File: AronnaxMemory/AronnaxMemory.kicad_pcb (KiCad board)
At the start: 6 copper layers, 161.3 x 64.8 mm, 38 parts, among them J1 Barrel_Jack_Switch, J11 Conn_02x18_Odd_Even, J2 Conn_02x40_Odd_Even, J3 Conn_02x18_Odd_Even, J8 RAM Select, J9 VP A1-A4, U10 AS6C4008-55PCN, U11 AS6C4008-55PCN, U12 AS6C4008-55PCN, U2 ATF22V10, U3 ATF22V10, U4 74AHCT32, U5 74HC74, U8 74HC74, U9 AS6C4008-55PCN, X1 16MHz

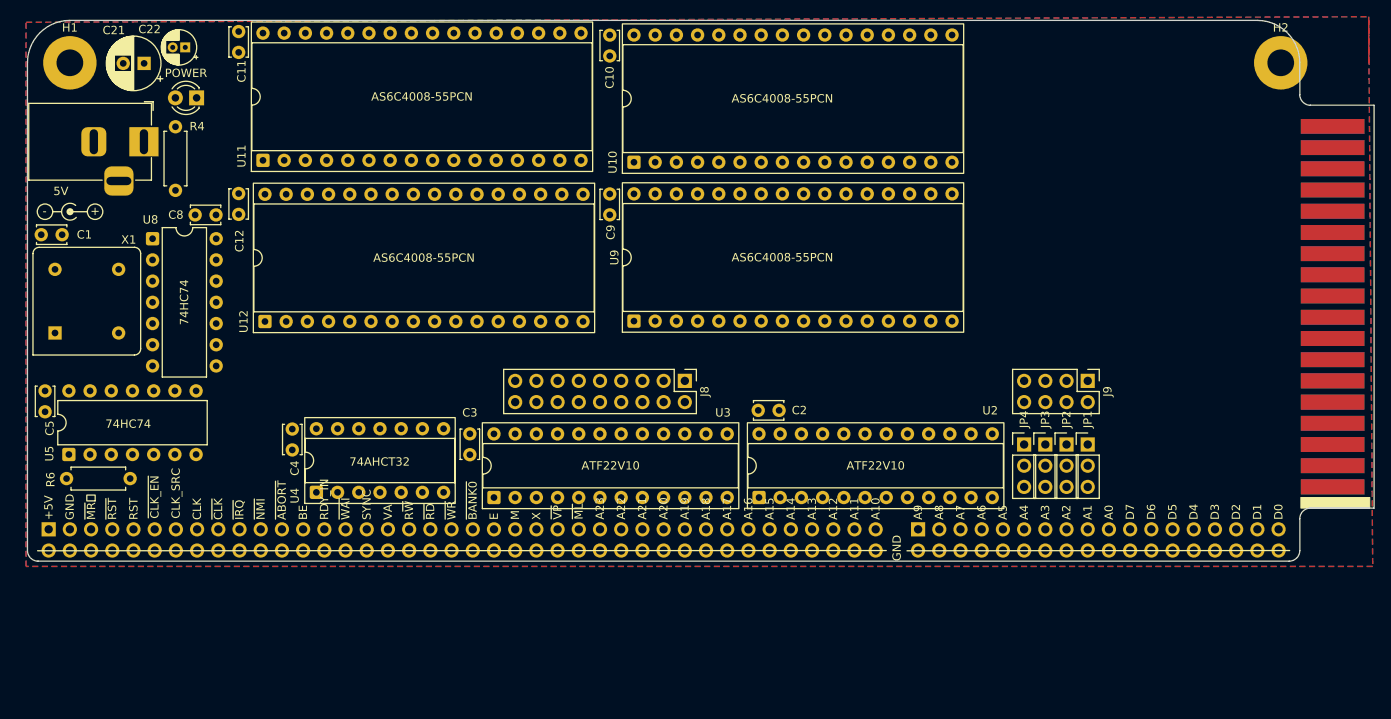
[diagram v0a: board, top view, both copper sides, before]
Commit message: May 2025
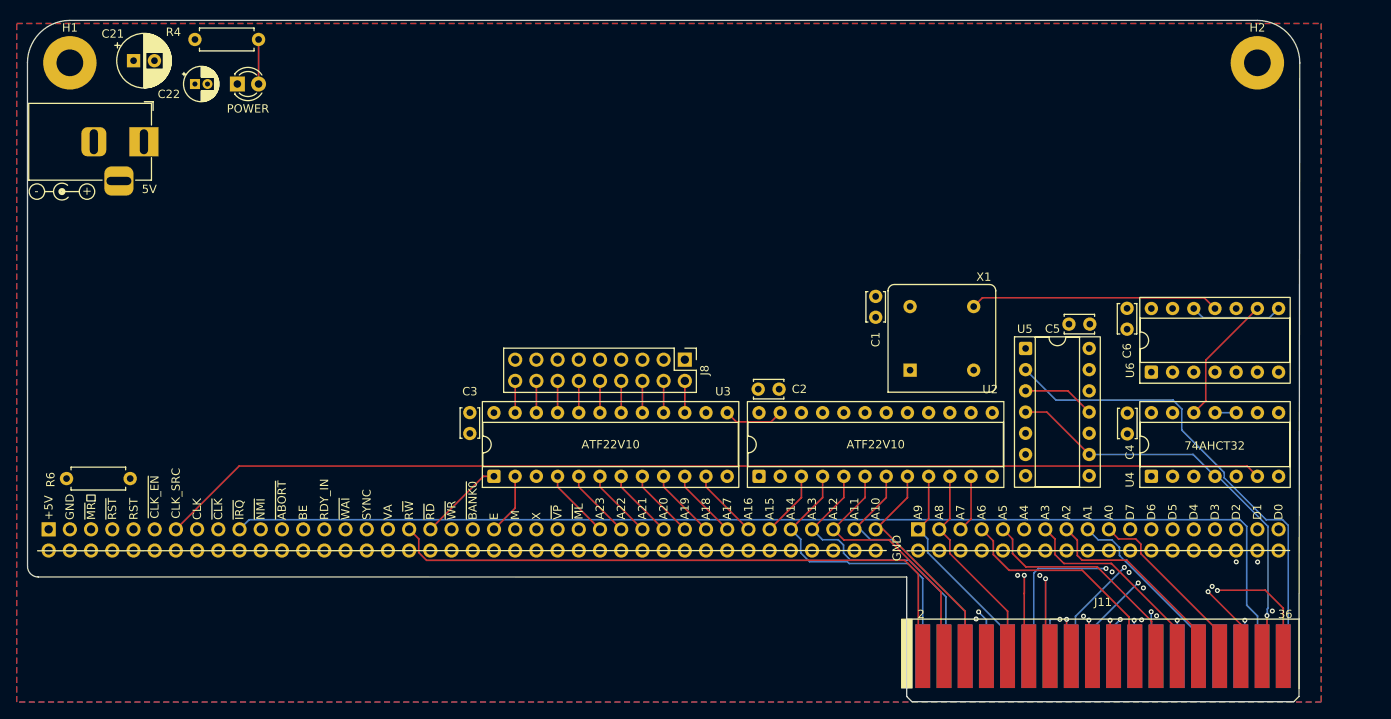
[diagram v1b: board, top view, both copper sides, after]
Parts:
- removed C10, C11, C12, C8, C9: 100nF, Capacitor_THT:C_Disc_D3.4mm_W2.1mm_P2.50mm
- removed J9: VP A1-A4, Connector_PinHeader_2.54mm:PinHeader_2x04_P2.54mm_Vertical
- removed JP1, JP2, JP3, JP4: Jumper3_254mm, Jumper3_254mm:Jumper3_254mm
- removed U10, U11, U12, U9: AS6C4008-55PCN, Package_DIP:DIP-32_W15.24mm_Socket
- removed U8: 74HC74, Package_DIP:DIP-14_W7.62mm
- added C6: 100nF, Capacitor_THT:C_Disc_D3.4mm_W2.1mm_P2.50mm, F.Cu at (157.1, 100.5)
- added U6: 74HC74, Package_DIP:DIP-14_W7.62mm_Socket, F.Cu at (160.0, 108.2)
- J11: moved to F.Cu
- U5: footprint Package_DIP:DIP-14_W7.62mm -> Package_DIP:DIP-14_W7.62mm_Socket
- moved C5 125.4 mm to (152.7, 102.4), turned to 180 degrees
- moved U5 115.3 mm to (145.0, 105.3), turned to 0 degrees
- moved X1 102.5 mm to (131.1, 107.9)
- moved C1 100.2 mm to (127.0, 99.1), turned to -90 degrees
- moved U4 100.0 mm to (160.0, 120.7)
- moved C4 100.0 mm to (157.1, 113.1)
- moved J11 49.1 mm to (154.2, 136.5), turned to 0 degrees
- moved R4 14.4 mm to (53.1, 68.3), turned to 180 degrees
- moved D1 5.16 mm to (50.5, 73.7), turned to 0 degrees
- moved C22 4.54 mm to (45.5, 73.7), turned to 0 degrees
- moved H2 2.80 mm to (172.7, 71.1)
- moved REF** 2.60 mm to (29.5, 86.5)
- moved C2 2.54 mm to (112.9, 110.2)
- moved C3 2.54 mm to (78.4, 113.0)
- moved J8 2.54 mm to (104.1, 106.7)
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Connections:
- U2 pad 10: /A7 -> /A8
- U2 pad 11: /~{BANK0} -> /A7
- U2 pad 13: /~{VP} -> unconnected-(U2-I-Pad13)
- U2 pad 14: /E -> unconnected-(U2-O-Pad14)
- U2 pad 2: /A15 -> /~{BANK0}
- U2 pad 22: /~{VPR} -> unconnected-(U2-O-Pad22)
- U2 pad 3: /A14 -> /A15
- U2 pad 4: /A13 -> /A14
- U2 pad 5: /A12 -> /A13
- U2 pad 6: /A11 -> /A12
- U2 pad 7: /A10 -> /A11
- U2 pad 8: /A9 -> /A10
- U2 pad 9: /A8 -> /A9
- U3 pad 1: GND -> /~{RD}
- U3 pad 13: GND -> /IO_AREA
- U3 pad 2: /IO_AREA -> /E
- U3 pad 3: /~{RD} -> GND
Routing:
- net /~{RESET}: track 0.00 -> 152.2 mm, vias 0 -> 1
- net /~{IRQ}: track 0.00 -> 137.8 mm
- net /CLK_SRC: track 0.00 -> 133.2 mm
- net /~{NMI}: track 0.00 -> 127.0 mm, vias 0 -> 1
- net /R~{W}: track 0.00 -> 74.2 mm
- net /~{IOREADY}: track 0.00 -> 57.0 mm
- net /IOWAIT: track 0.00 -> 50.6 mm, vias 0 -> 1
- net /IO_AREA: track 0.00 -> 46.3 mm
- net /~{BANK0}: track 0.00 -> 39.5 mm
- net /A7: track 0.00 -> 37.8 mm, vias 0 -> 1
- net /A14: track 0.00 -> 36.4 mm
- net /A13: track 0.00 -> 35.1 mm
- net /D0: track 0.00 -> 33.9 mm, vias 0 -> 1
- net /D3: track 0.00 -> 32.9 mm, vias 0 -> 1
- net /DCLK: track 0.00 -> 32.2 mm
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- added copper zone on In3.Cu, net GND
- added copper zone on In4.Cu, net GND
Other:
- board size 161.3 x 64.8 mm -> 152.4 x 81.6 mm
